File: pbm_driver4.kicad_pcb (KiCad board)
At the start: 4 copper layers, 65 x 150 mm, 113 parts, among them Q1 PSMN4R0-30YLD, Q2 PSMN4R0-30YLD, Q3 PSMN4R0-30YLD, Q4 PSMN4R0-30YLD, Q5 PSMN4R0-30YLD, Q6 PSMN4R0-30YLD, Q7 PSMN4R0-30YLD, Q8 PSMN4R0-30YLD, Q9 MMBT3906, U1 ADA4099-2, U10 TMUX1112PWR, U11 TMUX1112PWR, U12 D36V6F5, U2 ADA4099-2, U3 ADA4099-2, U4 ADA4099-2, U5 STM32G431RBTx, U6 LP2985-3.3, U8 TMP422

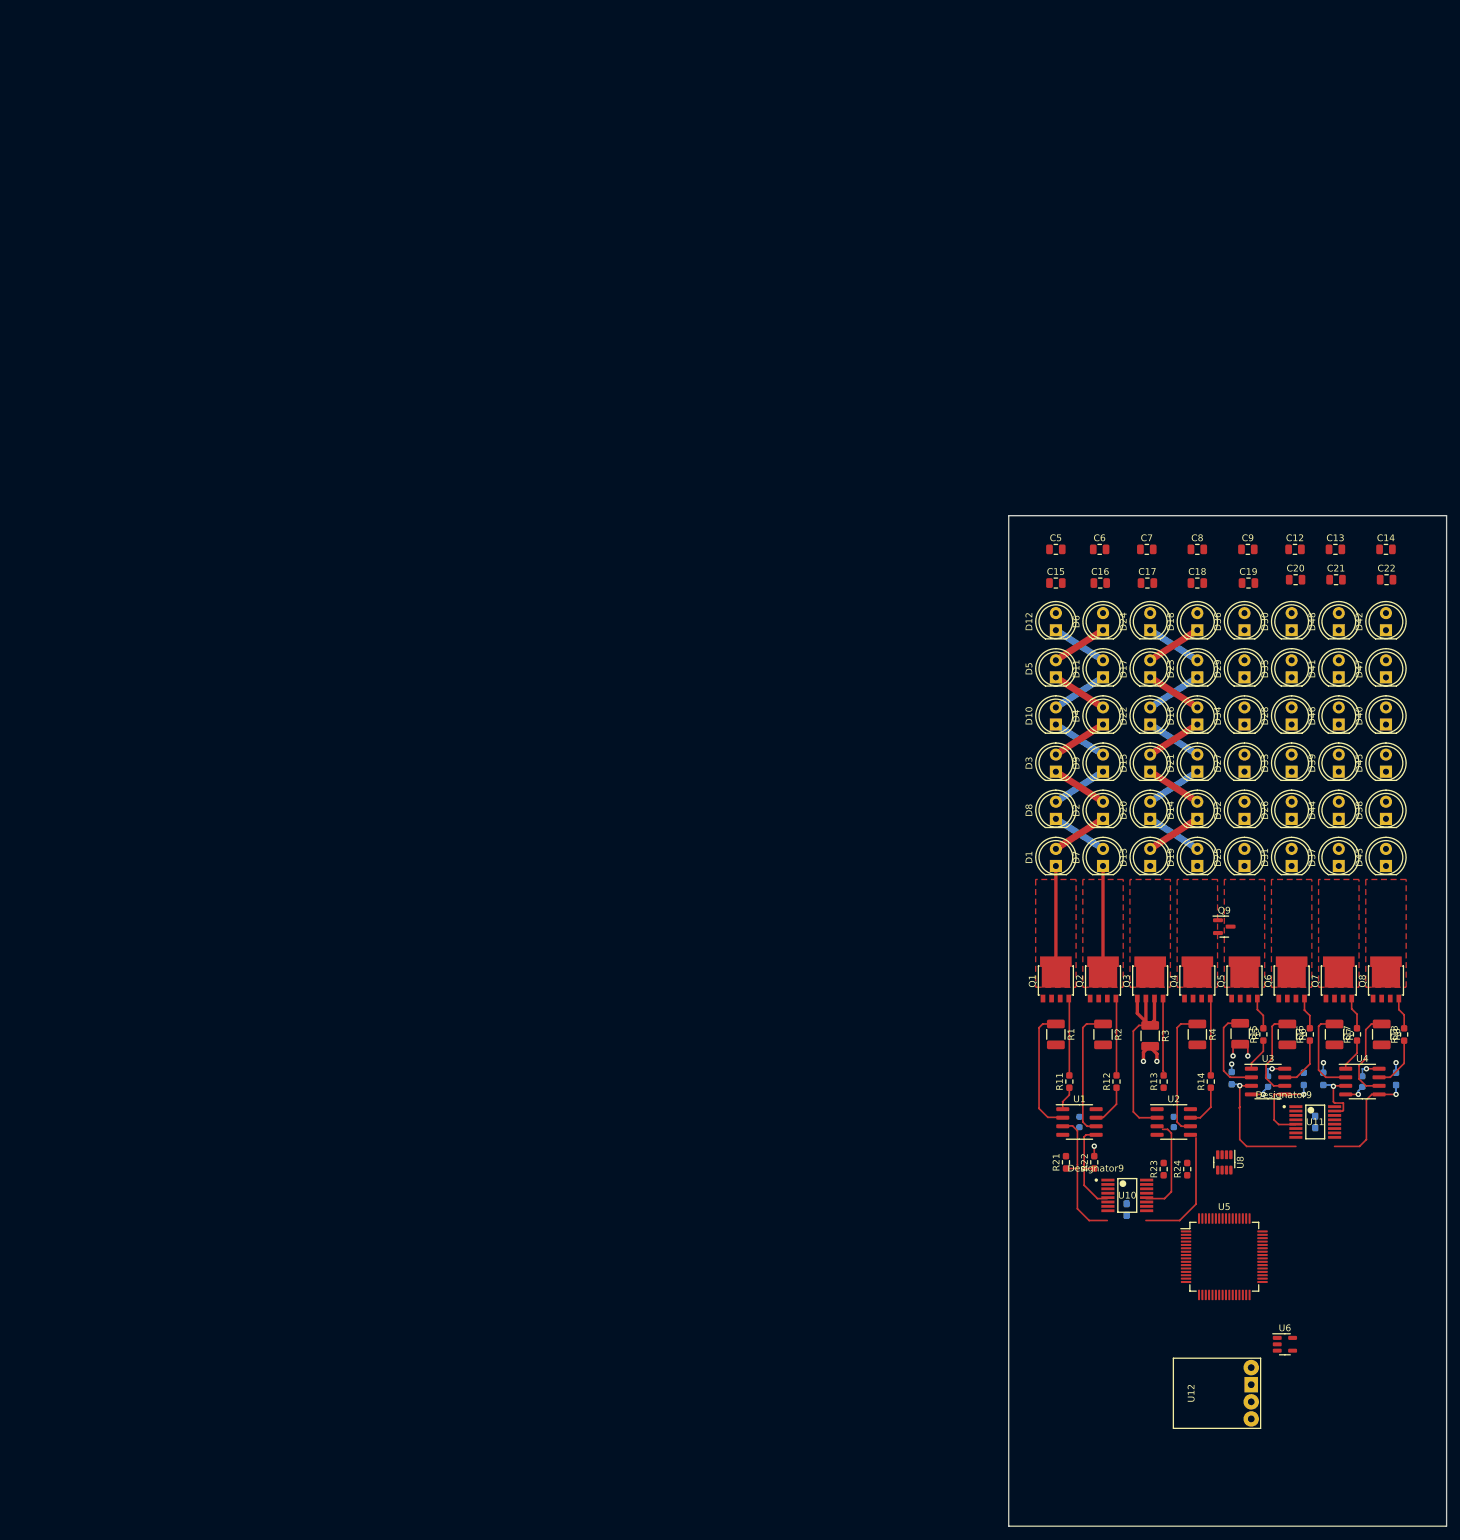
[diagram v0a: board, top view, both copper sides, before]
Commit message: As released to fab PCB103_RevA
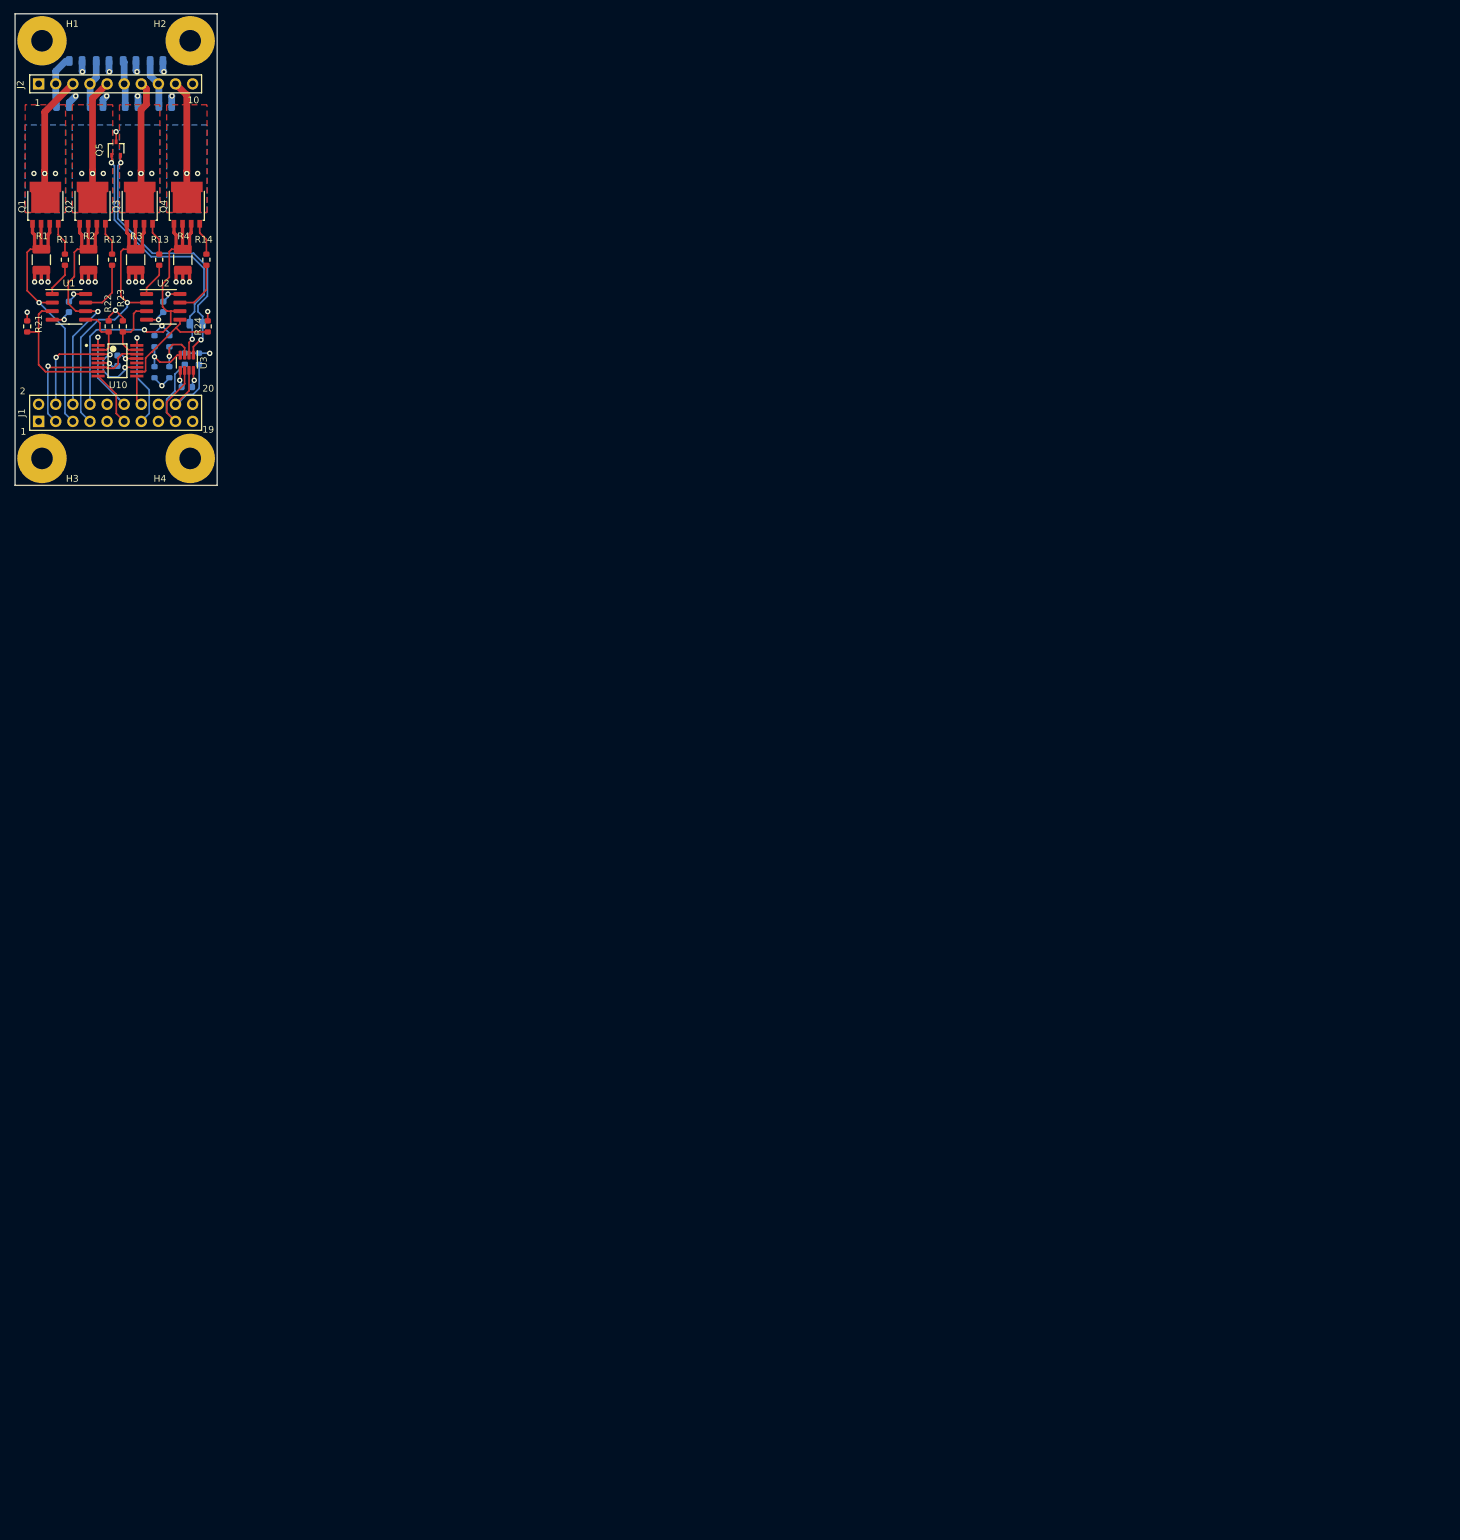
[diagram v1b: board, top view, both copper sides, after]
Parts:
- removed C14, C15, C16, C17, C18, C19, C20, C21, C22: 10uF, Capacitor_SMD:C_0805_2012Metric
- removed D1, D13, D14, D15, D16, D17, D18, D2, D25, D26, D27, D28, D29, D3, D30, D37, D38, D39, D4, D40, D41, D42, D5, D6: VSLY5850, LED_THT:LED_D5.0mm
- removed D10, D11, D12, D19, D20, D21, D22, D23, D24, D31, D32, D33, D34, D35, D36, D43, D44, D45, D46, D47, D48, D7, D8, D9: TLDR5800, LED_THT:LED_D5.0mm
- removed Q6, Q7, Q8: PSMN4R0-30YLD, Package_TO_SOT_SMD:LFPAK56
- removed Q9: MMBT3906, Package_TO_SOT_SMD:SOT-23
- removed R15, R16, R17, R18: 100, Resistor_SMD:R_0603_1608Metric_Pad0.98x0.95mm_HandSolder
- removed R25, R26, R27, R28: 100K, Resistor_SMD:R_0603_1608Metric_Pad0.98x0.95mm_HandSolder
- removed U11: TMUX1112PWR, $Local:PW0016A-IPC_A
- removed U12: D36V6F5, $Local:D36V6F5
- removed U4: ADA4099-2, Package_SO:SOIC-8_3.9x4.9mm_P1.27mm
- removed U5: STM32G431RBTx, Package_QFP:LQFP-64_10x10mm_P0.5mm
- removed U6: LP2985-3.3, Package_TO_SOT_SMD:SOT-23-5
- removed U8: TMP422, Package_TO_SOT_SMD:SOT-23-8
- added H1: MountingHole_Pad, $Local:MountingHole_3.2mm_M3_Pad, F.Cu at (6.50, -60.5)
- added H2: MountingHole_Pad, $Local:MountingHole_3.2mm_M3_Pad, F.Cu at (28.5, -60.5)
- added H3: MountingHole_Pad, $Local:MountingHole_3.2mm_M3_Pad, F.Cu at (6.50, 1.50)
- added H4: MountingHole_Pad, $Local:MountingHole_3.2mm_M3_Pad, F.Cu at (28.5, 1.50)
- added J1: Conn_02x10_Odd_Even, $Local:PinHeader_2x10_P2.54mm_Vertical, F.Cu at (6.00, -4.00)
- added J2: Conn_01x10, $Local:PinHeader_1x10_P2.54mm_Vertical, F.Cu at (6.00, -54.1)
- added R10: 10K, $Local:R_0603_1608Metric, B.Cu at (27.7, -13.3)
- added R9: 10K, $Local:R_0603_1608Metric, B.Cu at (29.8, -13.3)
- C1, C2, C3: value 1nF -> 0.1uF; footprint Capacitor_SMD:C_0603_1608Metric -> $Local:C_0603_1608Metric
- C10: value 1nF -> 0.1uF; footprint Capacitor_SMD:C_0603_1608Metric_Pad1.08x0.95mm_HandSolder -> $Local:C_0603_1608Metric
- C11: value 1nF -> 10uF; footprint Capacitor_SMD:C_0603_1608Metric_Pad1.08x0.95mm_HandSolder -> $Local:C_0805_2012Metric
- C12, C5, C6, C7, C8, C9: footprint Capacitor_SMD:C_0805_2012Metric -> $Local:C_0805_2012Metric; moved to B.Cu
- C13: value 10uF -> 100pF; footprint Capacitor_SMD:C_0805_2012Metric -> $Local:C_0805_2012Metric; moved to B.Cu
- C4: value 1nF -> 10uF; footprint Capacitor_SMD:C_0603_1608Metric -> $Local:C_0805_2012Metric
- Q1, Q2, Q3, Q4: footprint Package_TO_SOT_SMD:LFPAK56 -> $Local:LFPAK56
- Q5: value PSMN4R0-30YLD -> MMBT3906; footprint Package_TO_SOT_SMD:LFPAK56 -> $Local:SOT-323_SC-70
- R1, R2, R3, R4: footprint Resistor_SMD:R_1210_3225Metric_Pad1.30x2.65mm_HandSolder -> $Local:R_1210_3225Metric_Pad1.30x2.65mm_HandSolder
- R11, R12, R13, R14, R21, R22, R23, R24: footprint Resistor_SMD:R_0603_1608Metric_Pad0.98x0.95mm_HandSolder -> $Local:R_0603_1608Metric
- R5, R6, R7, R8: value 0.510 -> 10K; footprint Resistor_SMD:R_1210_3225Metric_Pad1.30x2.65mm_HandSolder -> $Local:R_0603_1608Metric; moved to B.Cu
- U1, U2: footprint Package_SO:SOIC-8_3.9x4.9mm_P1.27mm -> $Local:SOIC-8_3.9x4.9mm_P1.27mm
- U3: value ADA4099-2 -> TMP421; footprint Package_SO:SOIC-8_3.9x4.9mm_P1.27mm -> $Local:SOT-23-8
- moved C4 243.8 mm to (11.5, -57.5), turned to 0 degrees
- moved C11 233.2 mm to (23.5, -57.5), turned to 0 degrees
- moved R8 209.2 mm to (23.2, -15.9), turned to 90 degrees
- moved Q5 208.1 mm to (17.5, -44.5)
- moved R7 200.9 mm to (23.2, -11.3), turned to 90 degrees
- moved R23 198.8 mm to (18.5, -18.1)
- moved R21 197.9 mm to (4.30, -18.1)
- moved C10 195.7 mm to (17.7, -13.0)
- moved R6 195.3 mm to (25.4, -15.9), turned to 90 degrees
- moved U10 194.5 mm to (17.7, -13.0)
- moved U3 192.7 mm to (28.0, -12.7), turned to -90 degrees
- moved C1 192.7 mm to (10.5, -21.0)
- moved C2 192.7 mm to (24.5, -21.0)
- moved U1 192.7 mm to (10.5, -21.0)
- moved U2 192.7 mm to (24.5, -21.0)
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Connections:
- C11 pad 1: +3.3V -> +12V
- C13 pad 1: +12V -> /Sheet 5/DX_P
- C13 pad 2: GND -> /Sheet 5/DX_N
- C3 pad 1: +12V -> +3.3V
- Q5 pad 1: /SENSE5 -> /Sheet 5/DX_N
- Q5 pad 2: /SENSE5 -> /Sheet 5/DX_P
- Q5 pad 3: /SENSE5 -> GND
- R5 pad 1: /SENSE5 -> +3.3V
- R5 pad 2: GND -> /Sheet 5/A1
- R6 pad 1: /SENSE6 -> /Sheet 5/A1
- R7 pad 1: /SENSE7 -> +3.3V
- R7 pad 2: GND -> /Sheet 5/A0
- R8 pad 1: /SENSE8 -> /Sheet 5/A0
- U3 pad 1: Net-(R15-Pad1) -> /Sheet 5/DX_P
- U3 pad 2: /SENSE5 -> /Sheet 5/DX_N
- U3 pad 3: /Sheet 3/REF1 -> /Sheet 5/A1
- U3 pad 4: GND -> /Sheet 5/A0
- U3 pad 5: /Sheet 3/REF2 -> GND
- U3 pad 6: /SENSE6 -> /I2C_SCL
- U3 pad 7: Net-(R16-Pad1) -> /I2C_SDA
- U3 pad 8: +12V -> +3.3V
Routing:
- net /Sheet 5/DX_P: track 0.00 -> 40.4 mm, vias 0 -> 2
- net /Sheet 5/DX_N: track 0.00 -> 40.0 mm, vias 0 -> 2
- net GND: track 23.2 -> 58.3 mm, vias 10 -> 29
- net /SENSE4: track 19.5 -> 50.2 mm, vias 0 -> 1
- net +12V: track 7.20 -> 34.9 mm
- net /SENSE1: track 18.9 -> 43.7 mm, vias 0 -> 1
- net /DAC2: track 0.00 -> 24.3 mm, vias 0 -> 3
- net /DAC1: track 0.00 -> 23.4 mm, vias 0 -> 1
- net /SENSE2: track 19.5 -> 42.0 mm, vias 0 -> 1
- net /Sheet 3/REF1: track 20.0 -> 0.00 mm, vias 1 -> 0
- net /I2C_SCL: track 0.00 -> 19.8 mm
- net /LED4: track 0.00 -> 18.2 mm, vias 0 -> 3
- net /LED3: track 0.00 -> 17.9 mm, vias 0 -> 3
- net /Sheet 3/REF4: track 17.2 -> 0.00 mm, vias 1 -> 0
- net /SENSE3: track 31.4 -> 47.2 mm, vias 0 -> 1
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- added copper zone on In2.Cu, net +12V
- added copper zone on In2.Cu, net +3.3V
- added copper zone on B.Cu, net /LED1
- added copper zone on B.Cu, net /LED2
- added copper zone on B.Cu, net /LED3
- added copper zone on B.Cu, net /LED4
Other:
- board size 65 x 150 mm -> 30 x 70 mm
- board text added: "1"
- board text added: "10"
- board text added: "19"
- board text added: "2"
- board text added: "20"
